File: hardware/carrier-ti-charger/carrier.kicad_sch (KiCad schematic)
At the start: 0 parts

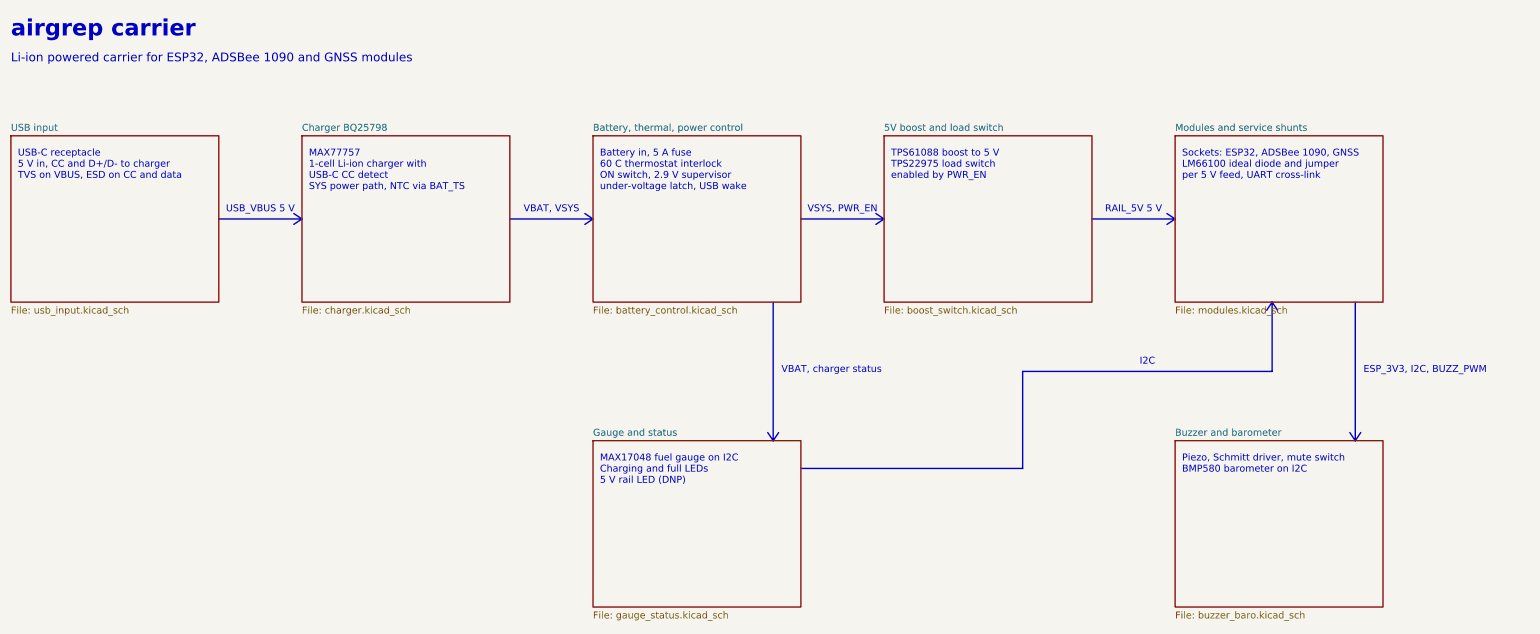
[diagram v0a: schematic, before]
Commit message: Other MH's.
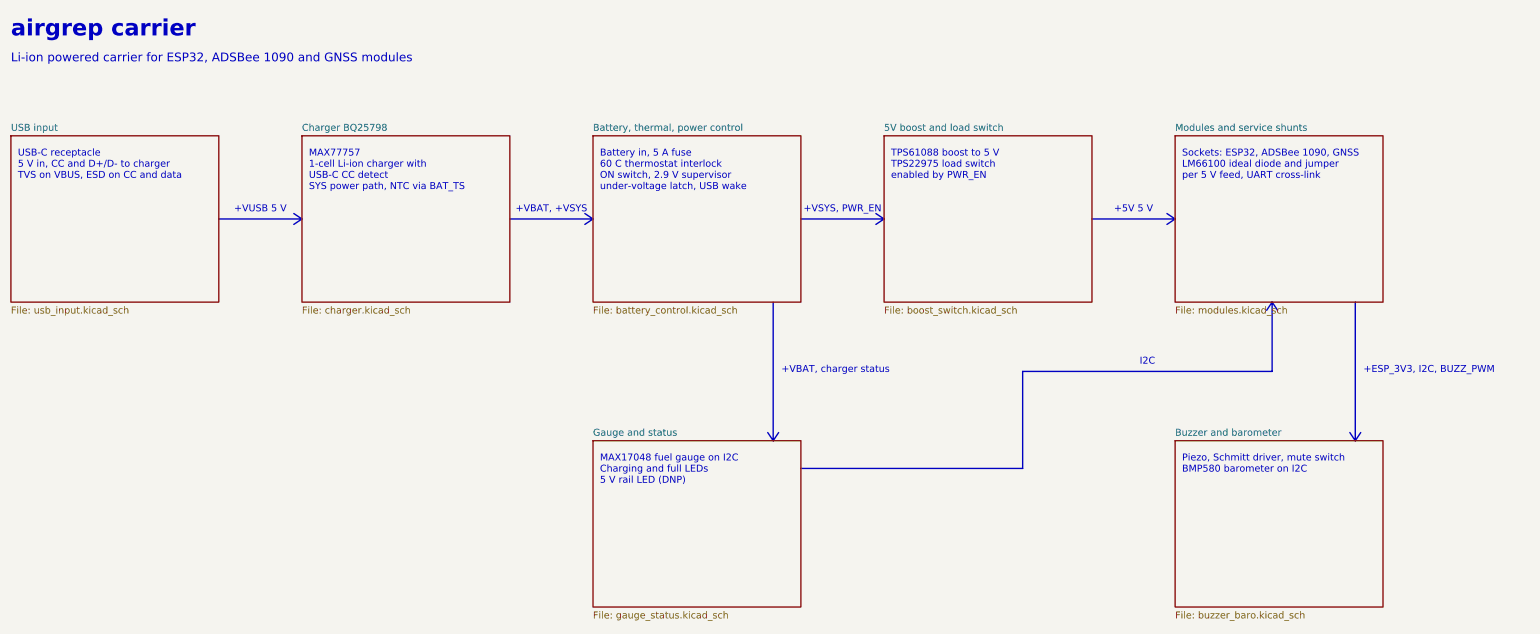
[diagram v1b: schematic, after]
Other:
- note added: "+5V 5 V"
- note added: "+ESP_3V3, I2C, BUZZ_PWM"
- note added: "+VBAT, +VSYS"
- note added: "+VBAT, charger status"
- note added: "+VSYS, PWR_EN"
- note added: "+VUSB 5 V"
- note removed: "ESP_3V3, I2C, BUZZ_PWM"
- note removed: "RAIL_5V 5 V"
- note removed: "USB_VBUS 5 V"
- note removed: "VBAT, VSYS"
- note removed: "VBAT, charger status"
- note removed: "VSYS, PWR_EN"
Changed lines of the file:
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@@
 		)
 	)
-	(text "VBAT, VSYS"
+	(text "+VBAT, +VSYS"
 		(exclude_from_sim no)
 		(at 119.38 65.04 0)
@@
 		)
 	)
-	(text "ESP_3V3, I2C, BUZZ_PWM"
+	(text "+ESP_3V3, I2C, BUZZ_PWM"
 		(exclude_from_sim no)
 		(at 268.2 94.48 0)
@@
 		)
 	)
-	(text "VBAT, charger status"
+	(text "+VBAT, charger status"
 		(exclude_from_sim no)
 		(at 161.52 94.48 0)
@@
 		)
 	)
-	(text "USB_VBUS 5 V"
+	(text "+VUSB 5 V"
 		(exclude_from_sim no)
 		(at 66.04 65.04 0)
@@
 		)
 	)
-	(text "RAIL_5V 5 V"
+	(text "+5V 5 V"
 		(exclude_from_sim no)
 		(at 226.06 65.04 0)
@@
 		)
 	)
-	(text "VSYS, PWR_EN"
+	(text "+VSYS, PWR_EN"
 		(exclude_from_sim no)
 		(at 172.72 65.04 0)
@@
 		(stroke
 			(width 0.254)
-			(type default)
+			(type solid)
+			(color 255 14 25 1)
 		)
 	)
@@
 		(stroke
 			(width 0.254)
-			(type default)
+			(type solid)
+			(color 255 14 25 1)
 		)
 	)
@@
 		(stroke
 			(width 0.254)
-			(type default)
+			(type solid)
+			(color 255 14 25 1)
 		)
 	)
@@
 		(stroke
 			(width 0.254)
-			(type default)
+			(type solid)
+			(color 255 14 25 1)
 		)
 	)
@@
 		(stroke
 			(width 0.254)
-			(type default)
-		)
-	)
+			(type solid)
+			(color 255 14 25 1)
+		)
+	)
